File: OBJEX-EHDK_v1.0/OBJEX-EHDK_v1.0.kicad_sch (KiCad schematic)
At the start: 4 parts

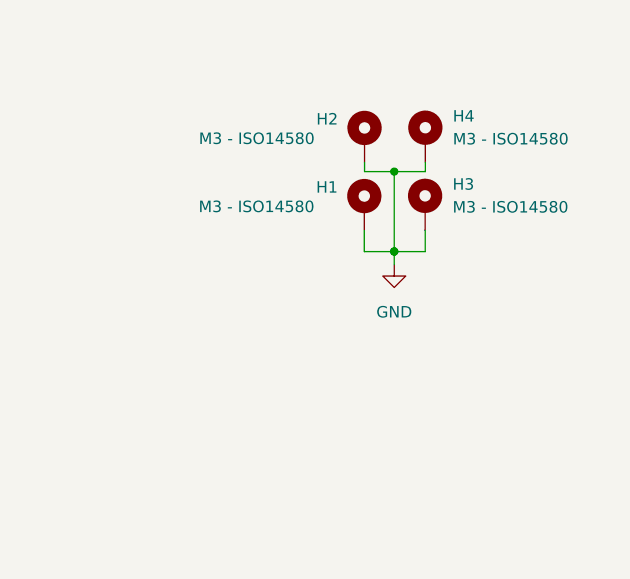
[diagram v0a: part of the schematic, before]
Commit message: SCH first review
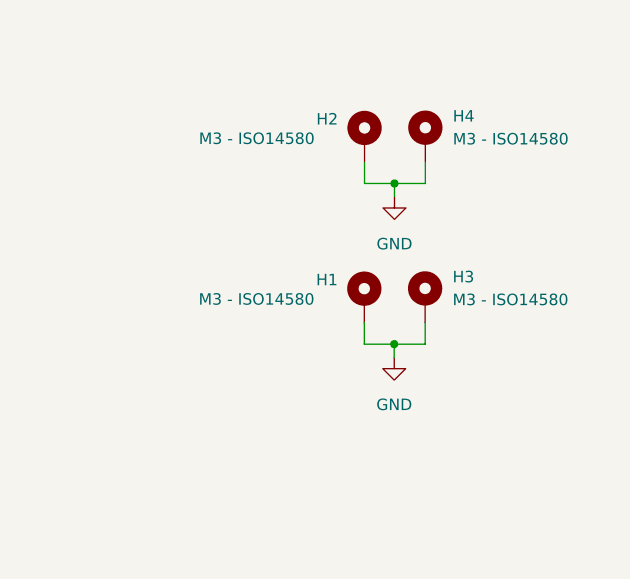
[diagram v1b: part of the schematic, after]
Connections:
- net GND: now also H2.1, H4.1
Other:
- moved on the sheet: H1, H3
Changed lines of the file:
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@@
     (comment 1 "Designer: Salvatore Raccardi")
   )
-  (junction (at 245.3894 96.647) (diameter 0) (color 0 0 0 0)
-  )
-  (junction (at 245.3894 96.6724) (diameter 0) (color 0 0 0 0)
-  )
-  (junction (at 245.3894 87.7824) (diameter 0) (color 0 0 0 0)
+  (junction (at 245.3894 106.9594) (diameter 0) (color 0 0 0 0)
+  )
+  (junction (at 245.4148 89.1032) (diameter 0) (color 0 0 0 0)
   )
   (wire (pts (xy 119.761 99.6696) (xy 126.0094 99.6696))
     (stroke (width 0) (type default) (color 0 0 0 0))
   )
-  (wire (pts (xy 245.3894 96.647) (xy 245.3894 87.7824))
-    (stroke (width 0) (type default) (color 0 0 0 0))
-  )
-  (wire (pts (xy 245.3894 96.6724) (xy 245.3894 98.1202))
-    (stroke (width 0) (type default) (color 0 0 0 0))
-  )
-  (wire (pts (xy 242.062 96.6724) (xy 245.3894 96.6724))
+  (wire (pts (xy 245.4148 89.1032) (xy 248.8438 89.1032))
+    (stroke (width 0) (type default) (color 0 0 0 0))
+  )
+  (wire (pts (xy 242.0874 89.1032) (xy 245.4148 89.1032))
+    (stroke (width 0) (type default) (color 0 0 0 0))
+  )
+  (wire (pts (xy 245.3894 106.9594) (xy 245.3894 108.4072))
+    (stroke (width 0) (type default) (color 0 0 0 0))
+  )
+  (wire (pts (xy 242.062 106.9594) (xy 245.3894 106.9594))
     (stroke (width 0) (type default) (color 0 0 0 0))
   )
@@
     (stroke (width 0) (type default) (color 0 0 0 0))
   )
-  (wire (pts (xy 248.8184 96.6724) (xy 248.8184 94.2848))
-    (stroke (width 0) (type default) (color 0 0 0 0))
-  )
-  (wire (pts (xy 242.062 94.3102) (xy 242.062 96.6724))
+  (wire (pts (xy 248.8184 106.9594) (xy 248.8184 104.5718))
+    (stroke (width 0) (type default) (color 0 0 0 0))
+  )
+  (wire (pts (xy 242.062 104.5972) (xy 242.062 106.9594))
     (stroke (width 0) (type default) (color 0 0 0 0))
   )
@@
     (stroke (width 0) (type default) (color 0 0 0 0))
   )
-  (wire (pts (xy 245.3894 96.6724) (xy 248.8184 96.6724))
-    (stroke (width 0) (type default) (color 0 0 0 0))
-  )
-  (wire (pts (xy 245.3894 87.7824) (xy 242.0874 87.7824))
-    (stroke (width 0) (type default) (color 0 0 0 0))
-  )
-  (wire (pts (xy 248.8438 87.7824) (xy 248.8438 86.7156))
+  (wire (pts (xy 245.3894 106.9594) (xy 248.8184 106.9594))
+    (stroke (width 0) (type default) (color 0 0 0 0))
+  )
+  (wire (pts (xy 248.8438 89.1032) (xy 248.8438 86.7156))
     (stroke (width 0) (type default) (color 0 0 0 0))
   )
@@
     (stroke (width 0) (type default) (color 0 0 0 0))
   )
-  (wire (pts (xy 242.0874 87.7824) (xy 242.0874 86.741))
-    (stroke (width 0) (type default) (color 0 0 0 0))
-  )
-  (wire (pts (xy 245.3894 87.7824) (xy 248.8438 87.7824))
+  (wire (pts (xy 245.4148 89.1032) (xy 245.4148 90.551))
     (stroke (width 0) (type default) (color 0 0 0 0))
   )
   (wire (pts (xy 119.761 106.7816) (xy 136.4488 106.7816))
+    (stroke (width 0) (type default) (color 0 0 0 0))
+  )
+  (wire (pts (xy 242.0874 86.741) (xy 242.0874 89.1032))
     (stroke (width 0) (type default) (color 0 0 0 0))
   )
@@
     (effects (font (size 3.5 3.5) italic) (justify left bottom))
   )
-  (symbol (lib_id "power:GND") (at 245.3894 98.1202 0) (unit 1)
+  (symbol (lib_id "power:GND") (at 245.3894 108.4072 0) (unit 1)
     (in_bom yes) (on_board yes) (fields_autoplaced)
-    (property "Reference" "#PWR0136" (id 0) (at 245.3894 104.4702 0)
-      (effects (font (size 1.27 1.27)) hide)
-    )
-    (property "Value" "GND" (id 1) (at 245.3894 103.4034 0))
-    (property "Footprint" "" (id 2) (at 245.3894 98.1202 0)
-      (effects (font (size 1.27 1.27)) hide)
-    )
-    (property "Datasheet" "" (id 3) (at 245.3894 98.1202 0)
+    (property "Reference" "#PWR0136" (id 0) (at 245.3894 114.7572 0)
+      (effects (font (size 1.27 1.27)) hide)
+    )
+    (property "Value" "GND" (id 1) (at 245.3894 113.6904 0))
+    (property "Footprint" "" (id 2) (at 245.3894 108.4072 0)
+      (effects (font (size 1.27 1.27)) hide)
+    )
+    (property "Datasheet" "" (id 3) (at 245.3894 108.4072 0)
       (effects (font (size 1.27 1.27)) hide)
     )
     (pin "1")
   )
-  (symbol (lib_id "Mechanical:MountingHole_Pad") (at 242.062 91.7702 0) (unit 1)
+  (symbol (lib_id "Mechanical:MountingHole_Pad") (at 242.062 102.0572 0) (unit 1)
     (in_bom yes) (on_board yes)
-    (property "Reference" "H1" (id 0) (at 236.7026 89.535 0)
-      (effects (font (size 1.27 1.27)) (justify left))
-    )
-    (property "Value" "M3 - ISO14580" (id 1) (at 223.647 91.694 0)
-      (effects (font (size 1.27 1.27)) (justify left))
-    )
-    (property "Footprint" "MountingHole:MountingHole_3.2mm_M3_ISO14580_Pad" (id 2) (at 242.062 91.7702 0)
-      (effects (font (size 1.27 1.27)) hide)
-    )
-    (property "Datasheet" "~" (id 3) (at 242.062 91.7702 0)
+    (property "Reference" "H1" (id 0) (at 236.7026 99.822 0)
+      (effects (font (size 1.27 1.27)) (justify left))
+    )
+    (property "Value" "M3 - ISO14580" (id 1) (at 223.647 101.981 0)
+      (effects (font (size 1.27 1.27)) (justify left))
+    )
+    (property "Footprint" "MountingHole:MountingHole_3.2mm_M3_ISO14580_Pad" (id 2) (at 242.062 102.0572 0)
+      (effects (font (size 1.27 1.27)) hide)
+    )
+    (property "Datasheet" "~" (id 3) (at 242.062 102.0572 0)
       (effects (font (size 1.27 1.27)) hide)
     )
@@
     (pin "1")
   )
-  (symbol (lib_id "Mechanical:MountingHole_Pad") (at 248.8184 91.7448 0) (unit 1)
+  (symbol (lib_id "Mechanical:MountingHole_Pad") (at 248.8184 102.0318 0) (unit 1)
     (in_bom yes) (on_board yes) (fields_autoplaced)
-    (property "Reference" "H3" (id 0) (at 251.8664 89.2047 0)
-      (effects (font (size 1.27 1.27)) (justify left))
-    )
-    (property "Value" "M3 - ISO14580" (id 1) (at 251.8664 91.7447 0)
-      (effects (font (size 1.27 1.27)) (justify left))
-    )
-    (property "Footprint" "MountingHole:MountingHole_3.2mm_M3_ISO14580_Pad" (id 2) (at 248.8184 91.7448 0)
-      (effects (font (size 1.27 1.27)) hide)
-    )
-    (property "Datasheet" "~" (id 3) (at 248.8184 91.7448 0)
+    (property "Reference" "H3" (id 0) (at 251.8664 99.4917 0)
+      (effects (font (size 1.27 1.27)) (justify left))
+    )
+    (property "Value" "M3 - ISO14580" (id 1) (at 251.8664 102.0317 0)
+      (effects (font (size 1.27 1.27)) (justify left))
+    )
+    (property "Footprint" "MountingHole:MountingHole_3.2mm_M3_ISO14580_Pad" (id 2) (at 248.8184 102.0318 0)
+      (effects (font (size 1.27 1.27)) hide)
+    )
+    (property "Datasheet" "~" (id 3) (at 248.8184 102.0318 0)
       (effects (font (size 1.27 1.27)) hide)
     )
@@
     )
     (property "Datasheet" "~" (id 3) (at 248.8438 84.1756 0)
+      (effects (font (size 1.27 1.27)) hide)
+    )
+    (pin "1")
+  )
+  (symbol (lib_id "power:GND") (at 245.4148 90.551 0) (unit 1)
+    (in_bom yes) (on_board yes) (fields_autoplaced)
+    (property "Reference" "#PWR0138" (id 0) (at 245.4148 96.901 0)
+      (effects (font (size 1.27 1.27)) hide)
+    )
+    (property "Value" "GND" (id 1) (at 245.4148 95.8342 0))
+    (property "Footprint" "" (id 2) (at 245.4148 90.551 0)
+      (effects (font (size 1.27 1.27)) hide)
+    )
+    (property "Datasheet" "" (id 3) (at 245.4148 90.551 0)
       (effects (font (size 1.27 1.27)) hide)
     )
@@
       (reference "#PWR0137") (unit 1) (value "GND") (footprint "")
     )
+    (path "/e0fe93aa-01b7-4df1-8aae-5662e8118bb7"
+      (reference "#PWR0138") (unit 1) (value "GND") (footprint "")
+    )
     (path "/1bd0dc3d-4de3-423e-bb17-63b75cf64400/709ea27c-ada8-4cd1-83ef-6adacf2c94d1"
